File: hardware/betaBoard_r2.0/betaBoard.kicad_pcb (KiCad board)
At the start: 2 copper layers, 70 x 45 mm, 141 parts, among them J1 DNP, J2 AMPHENOL_10103592-0001LF, J3 DNP, J4 DNP, J5 DNP, J6 DNP, SW1 TS-1187A-B-A-B, SW2 TS-1187A-B-A-B, U1 AMS1117-3.3_SOT223, U2 W25Q128JVSIQ, U3 RP2040, U4 LM358, U5 LM358, U6 LM358, U7 LM358, Y1 X322512MSB4SI

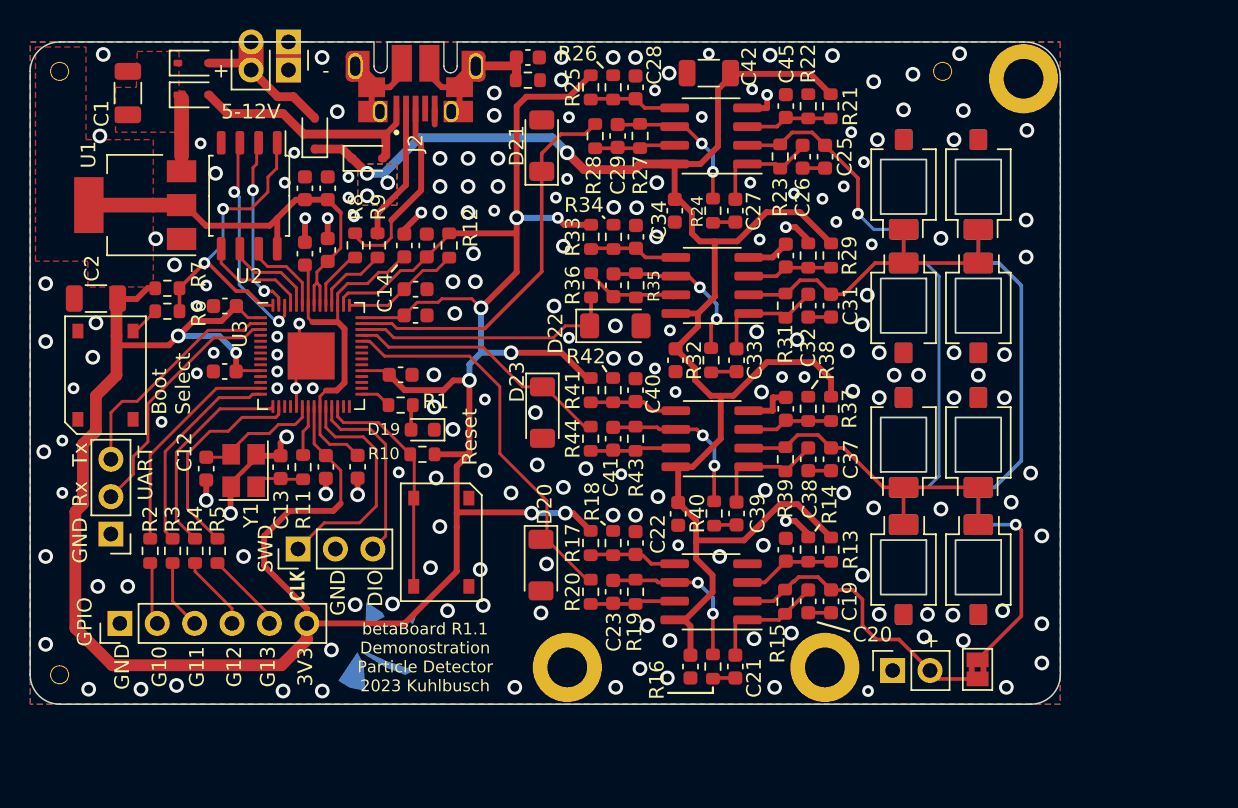
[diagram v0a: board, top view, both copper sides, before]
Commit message: main r2.0 design done
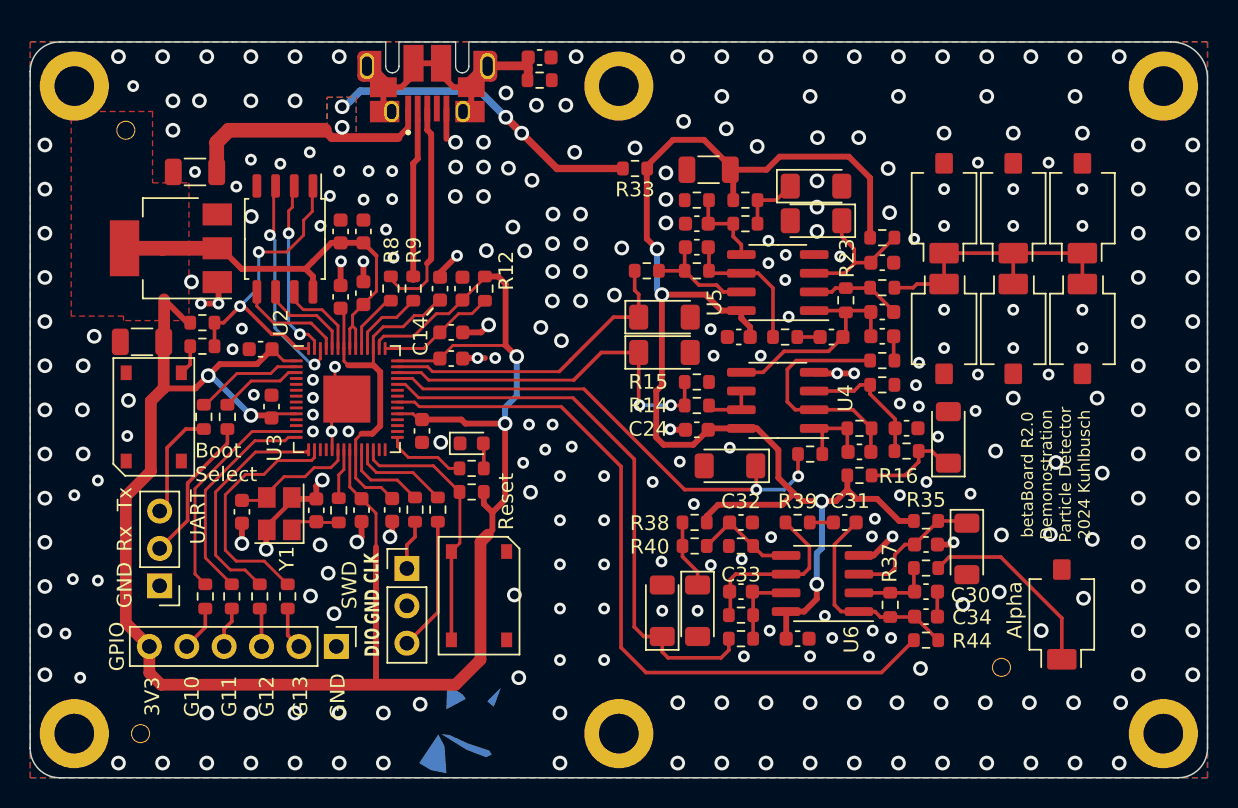
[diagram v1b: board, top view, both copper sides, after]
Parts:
- removed C35, C41: 47p, Capacitor_SMD:C_0603_1608Metric
- removed C36: 100n, Capacitor_SMD:C_0603_1608Metric
- removed C37, C38: 10p, Capacitor_SMD:C_0603_1608Metric
- removed C39: 470n, Capacitor_SMD:C_0603_1608Metric
- removed C40: 1u, Capacitor_SMD:C_0603_1608Metric
- removed C42: 10u, Capacitor_SMD:C_1206_3216Metric
- removed C44, C46, C47: 10u, Capacitor_SMD:C_0603_1608Metric
- removed D16: DNP, OptoDevice:Osram_BPW34S-SMD
- removed D17, D18, D24, D25: 1N5819WS, Diode_SMD:D_SOD-323
- removed D20, D22, D23: ZMM3V3-M, Diode_SMD:D_MiniMELF
- removed J1: DNP, betaBoard:PinHeader_1x02_P2.54mm_castellation
- removed J3: DNP, Connector_PinSocket_2.54mm:PinSocket_1x02_P2.54mm_Vertical
- removed JP1: DNP, Jumper:SolderJumper-2_P1.3mm_Bridged2Bar_Pad1.0x1.5mm
- removed U7: LM358, Package_SO:SOIC-8_3.9x4.9mm_P1.27mm
- added H7: M3 Hole, MountingHole:MountingHole_2.7mm_M2.5_DIN965_Pad, F.Cu at (90.0, 53.0)
- added H8: M3 Hole, MountingHole:MountingHole_2.7mm_M2.5_DIN965_Pad, F.Cu at (53.0, 97.0)
- added H9: M3 Hole, MountingHole:MountingHole_2.7mm_M2.5_DIN965_Pad, F.Cu at (53.0, 53.0)
- C1: value 10u -> 100u
- C19, C31: value 10p -> 100n
- C20, C32: value 10p -> 1u
- C21, C33: value 470n -> 10p
- C22: value 1u -> 100u; footprint Capacitor_SMD:C_0603_1608Metric -> Capacitor_SMD:C_1206_3216Metric
- C23: value 47p -> 100n
- C25: value 10p -> 10u
- C26: value 10p -> 2p2
- C27: value 470n -> 100n
- C29: value 47p -> 10p
- C30: value 100n -> 10p
- C34: value 1u -> 10p
- D1, D13, D5, D9: moved to F.Cu
- D10, D11, D14, D6, D7: value BPW34-SMD -> ZMM3V3-M; footprint betaBoard:Osram_BPW34S-SMD_hole -> Diode_SMD:D_MiniMELF
- D12, D4, D8: value DNP -> ZMM3V3-M; footprint OptoDevice:Osram_BPW34S-SMD -> Diode_SMD:D_MiniMELF; moved to F.Cu
- D15, D2, D3: value BPW34-SMD -> DNP; footprint betaBoard:Osram_BPW34S-SMD_hole -> OptoDevice:Osram_BPW34S-SMD
- R13, R21: value 47k -> 1k
- R14, R22, R30: value 150k -> 10k
- R15, R31: value 47M -> 10k
- R16, R24: value 4K7 -> 1k
- R17: value 10k -> 1k
- R19, R27: value 1M -> 100k
- R2, R3, R4, R5: value 1k -> 10k
- R23: value 47M -> 22M
- R26, R41, R42, R44: value 10k -> 100k
- R29: value 47k -> 10k
- R32, R40: value 4K7 -> 10k
- R33: value 10k -> 4R7
- R34, R36: value 10k -> 0
- R35: value 1M -> 1k
- R37: value 47k -> 10M
- R38: value 150k -> 1k
- R39: value 47M -> 1k
- R43: value 1M -> 10k
- R45: value 0 -> DNP
- U4, U5, U6: value LM358 -> MCP6232
- moved H6 75.7 mm to (116.0, 92.5)
- moved H5 70.7 mm to (57.5, 97.0)
- moved R31 40.2 mm to (61.8, 75.5), turned to -90 degrees
- moved H4 37.3 mm to (56.5, 56.0)
- moved R32 33.1 mm to (63.4, 75.5)
- moved C34 32.5 mm to (110.9, 89.0), turned to 180 degrees
- moved R30 31.8 mm to (76.2, 81.8), turned to -90 degrees
- moved R29 31.8 mm to (77.7, 81.8)
- moved R36 29.8 mm to (110.9, 85.8), turned to 0 degrees
- moved D12 28.1 mm to (95.3, 88.7)
- moved C25 27.2 mm to (110.9, 84.2), turned to 0 degrees
- moved R44 26.6 mm to (110.9, 90.7), turned to 0 degrees
- moved D14 26.3 mm to (93.0, 88.7), turned to 90 degrees
- moved C22 25.8 mm to (96.1, 58.7), turned to 180 degrees
- moved D5 25.7 mm to (116.8, 61.3), turned to 90 degrees
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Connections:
- C1 pad 1: /LDO_IN -> /5V_USB
- C19 pad 1: /particle_sensor_array/Diodes -> Net-(U4B-+)
- C20 pad 1: Net-(C19-Pad2) -> Net-(U4A-+)
- C20 pad 2: Net-(C20-Pad2) -> GND
- C21 pad 1: Net-(C20-Pad2) -> Net-(U4A--)
- C22 pad 1: Net-(U4B-+) -> VCC
- C23 pad 1: Net-(U4B--) -> VCC
- C23 pad 2: Net-(C23-Pad2) -> GND
- C25 pad 1: /particle_sensor_array1/Diodes -> Net-(D11-K)
- C25 pad 2: Net-(C25-Pad2) -> GND
- C26 pad 1: Net-(C25-Pad2) -> Net-(U5A--)
- C26 pad 2: Net-(C26-Pad2) -> Net-(U4B-+)
- C27 pad 1: Net-(C26-Pad2) -> Net-(U4B-+)
- C30 pad 1: VCC -> Net-(U6A--)
- C30 pad 2: GND -> Net-(C30-Pad2)
- C31 pad 1: /particle_sensor_array2/Diodes -> Net-(C31-Pad1)
- C32 pad 1: Net-(C31-Pad2) -> Net-(U6B-+)
- C32 pad 2: Net-(C32-Pad2) -> GND
- C33 pad 1: Net-(C32-Pad2) -> Net-(U6B--)
- C34 pad 1: Net-(U6B-+) -> Net-(C30-Pad2)
- C34 pad 2: GND -> Net-(C31-Pad1)
- C45 pad 1: Net-(U5A-+) -> Net-(D4-K)
- D10 pad 1: /particle_sensor_array2/Diodes -> /MCU/ADC1
- D11 pad 1: /particle_sensor_array3/Diodes -> Net-(D11-K)
- D14 pad 1: /particle_sensor_array2/Diodes -> /Frontend Alpha/out
- D15 pad 1: /particle_sensor_array3/Diodes -> /Frontend Alpha/Diodes
- D2 pad 1: /particle_sensor_array2/Diodes -> /particle_sensor_array1/Diodes
- D3 pad 1: /particle_sensor_array3/Diodes -> /particle_sensor_array1/Diodes
- D4 pad 1: Net-(D12-K) -> Net-(D4-K)
- D6 pad 1: /particle_sensor_array2/Diodes -> Net-(D6-K)
- D7 pad 1: /particle_sensor_array3/Diodes -> /MCU/ADC2
- D8 pad 1: Net-(D12-K) -> Net-(D8-K)
- J4 pad 2: /MCU/UART0_RX -> Net-(J4-Pin_2)
- J4 pad 3: /MCU/UART0_TX -> Net-(J4-Pin_3)
- J5 pad 1: /MCU/SWD_CLK -> Net-(J5-Pin_1)
- J5 pad 3: /MCU/SWD_SIO -> Net-(J5-Pin_3)
- R13 pad 2: Net-(U4A-+) -> Net-(D6-K)
- R14 pad 1: Net-(U4A-+) -> /MCU/ADC2
- R14 pad 2: GND -> Net-(U4B--)
- R15 pad 1: Net-(C20-Pad2) -> /MCU/ADC2
- R15 pad 2: /particle_sensor_array/Diodes -> GND
- R16 pad 1: Net-(U4B--) -> VCC
- R16 pad 2: Net-(C21-Pad2) -> Net-(D8-K)
- R17 pad 1: Net-(U4B-+) -> Net-(U4A--)
- R17 pad 2: +3V3 -> Net-(C19-Pad2)
- R18 pad 1: GND -> Net-(U4A-+)
- R18 pad 2: Net-(U4B-+) -> Net-(D8-K)
- R19 pad 1: Net-(C23-Pad2) -> GND
- R19 pad 2: Net-(U4B--) -> Net-(U4A-+)
- R2 pad 1: /MCU/GP10 -> /MCU/GP13
- R20 pad 1: /MCU/ADC0 -> Net-(C21-Pad2)
- R20 pad 2: Net-(C23-Pad2) -> Net-(U4A--)
- R21 pad 2: Net-(U5A-+) -> Net-(D4-K)
- R22 pad 1: Net-(U5A-+) -> /MCU/ADC1
- R22 pad 2: GND -> Net-(C21-Pad2)
- R23 pad 1: Net-(C26-Pad2) -> Net-(U4B-+)
- R23 pad 2: /particle_sensor_array1/Diodes -> Net-(U5A--)
- R25 pad 2: +3V3 -> Net-(D6-K)
- R29 pad 1: VCC -> /MCU/SWD_SIO
- R29 pad 2: Net-(U6A-+) -> Net-(J5-Pin_3)
- R3 pad 1: /MCU/GP11 -> /MCU/GP12
- R30 pad 1: Net-(U6A-+) -> /MCU/SWD_CLK
- R30 pad 2: GND -> Net-(J5-Pin_1)
- R31 pad 1: Net-(C32-Pad2) -> /MCU/UART0_TX
- R31 pad 2: /particle_sensor_array2/Diodes -> Net-(J4-Pin_3)
- R32 pad 1: Net-(U6B--) -> /MCU/UART0_RX
- R32 pad 2: Net-(C33-Pad2) -> Net-(J4-Pin_2)
- R33 pad 1: Net-(U6B-+) -> VCC
- R33 pad 2: +3V3 -> /5V_USB
- R34 pad 1: GND -> Net-(U5A--)
- R34 pad 2: Net-(U6B-+) -> /particle_sensor_array1/Diodes
- R35 pad 1: Net-(C35-Pad2) -> VCC
- R35 pad 2: Net-(U6B--) -> Net-(D11-K)
- R36 pad 1: /MCU/ADC2 -> Net-(U6A--)
- R36 pad 2: Net-(C35-Pad2) -> /Frontend Alpha/Diodes
- R37 pad 1: VCC -> Net-(C31-Pad1)
- R37 pad 2: Net-(U7A-+) -> Net-(U6A--)
- R38 pad 1: Net-(U7A-+) -> VCC
- R38 pad 2: GND -> Net-(D12-K)
- R39 pad 1: Net-(C38-Pad2) -> Net-(U6B--)
- R39 pad 2: /particle_sensor_array3/Diodes -> Net-(C31-Pad2)
- R4 pad 1: /MCU/GP12 -> /MCU/GP11
- R40 pad 1: Net-(U7B--) -> Net-(U6B-+)
- R40 pad 2: Net-(C39-Pad2) -> Net-(D12-K)
- R41 pad 1: Net-(U7B-+) -> GND
- R41 pad 2: +3V3 -> Net-(U6B-+)
- R42 pad 1: GND -> Net-(C33-Pad2)
- R42 pad 2: Net-(U7B-+) -> Net-(U6B--)
- R43 pad 1: Net-(C41-Pad2) -> /Frontend Alpha/out
- R43 pad 2: Net-(U7B--) -> Net-(C33-Pad2)
- R44 pad 1: /MCU/ADC1 -> /Frontend Alpha/out_bias
- R44 pad 2: Net-(C41-Pad2) -> Net-(C31-Pad1)
- R5 pad 1: /MCU/GP13 -> /MCU/GP10
- U1 pad 3: /LDO_IN -> /5V_USB
- U3 pad 35: unconnected-(U3-GPIO23-Pad35) -> /Frontend Alpha/out_bias
- U3 pad 38: /MCU/ADC0 -> /Frontend Alpha/out
- U4 pad 1: Net-(C20-Pad2) -> Net-(C21-Pad2)
- U4 pad 2: /particle_sensor_array/Diodes -> Net-(U4A--)
- U4 pad 7: Net-(C23-Pad2) -> Net-(U4B--)
- U5 pad 1: Net-(C26-Pad2) -> Net-(U4B-+)
- U5 pad 2: /particle_sensor_array1/Diodes -> Net-(U5A--)
- U5 pad 3: Net-(U5A-+) -> Net-(D4-K)
- U6 pad 1: Net-(C32-Pad2) -> Net-(C31-Pad1)
- U6 pad 2: /particle_sensor_array2/Diodes -> Net-(U6A--)
- U6 pad 3: Net-(U6A-+) -> Net-(D11-K)
- U6 pad 7: Net-(C35-Pad2) -> Net-(C33-Pad2)
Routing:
- net /Frontend Alpha/out_bias: track 0.00 -> 50.8 mm
- net +3V3: track 221.9 -> 172.4 mm, vias 9 -> 4
- net /Frontend Alpha/out: track 0.00 -> 38.5 mm
- net Net-(D12-K): track 37.1 -> 4.67 mm, vias 1 -> 0
- net VCC: track 120.5 -> 92.6 mm
- net /MCU/ADC0: track 26.5 -> 0.00 mm
- net /5V_USB: track 16.9 -> 39.8 mm, vias 0 -> 4
- net /particle_sensor_array3/Diodes: track 22.5 -> 0.00 mm
- net /particle_sensor_array2/Diodes: track 21.9 -> 0.00 mm
- net /particle_sensor_array/Diodes: track 20.2 -> 0.00 mm
- net /particle_sensor_array1/Diodes: track 38.8 -> 19.2 mm, vias 1 -> 0
- net /MCU/ADC1: track 17.6 -> 33.9 mm, vias 0 -> 2
- net Net-(U4A--): track 0.00 -> 16.2 mm
- net Net-(C31-Pad1): track 0.00 -> 14.3 mm
- net /Frontend Alpha/Diodes: track 0.00 -> 13.2 mm
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- added copper zone on B.Cu, net /5V_USB
- added copper zone on F.Cu, net /5V_USB
- removed copper zone on F.Cu, net /LDO_IN
- removed copper zone on B.Cu, net VCC
- removed copper zone on F.Cu, net VCC
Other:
- board size 70 x 45 mm -> 80 x 50 mm
- board text added: "Accepted DRC Error: - USB port: 3 errors - Boot Select button: 1 error"
- board text added: "Alpha"
- board text added: "betaBoard R2.0 Demonostration Particle Detector 2024 Kuhlbusch"
- board text removed: "+"
- board text removed: "-"
- board text removed: "5-12V"
- board text removed: "Castellations produce 2 errors in DRC"
- board text removed: "Details: https://github.com/timbk/BetaBoard"
- board text removed: "Unmarked 0603 are mostly 100nF"
- board text removed: "betaBoard R1.1 Demonostration Particle Detector 2023 Kuhlbusch"
